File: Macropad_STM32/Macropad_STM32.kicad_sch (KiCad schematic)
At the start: 68 parts, among them J1 USB_C_Receptacle_USB2.0, J10 Encoders + LED, J2 Conn_01x04_Pin, J3 JTAG, J7 Power Connector, J9 Matrix, SW1 SW_Push, U1 STM32F103C8T6, U3 AMS1117-3.3, Y1 16MHz

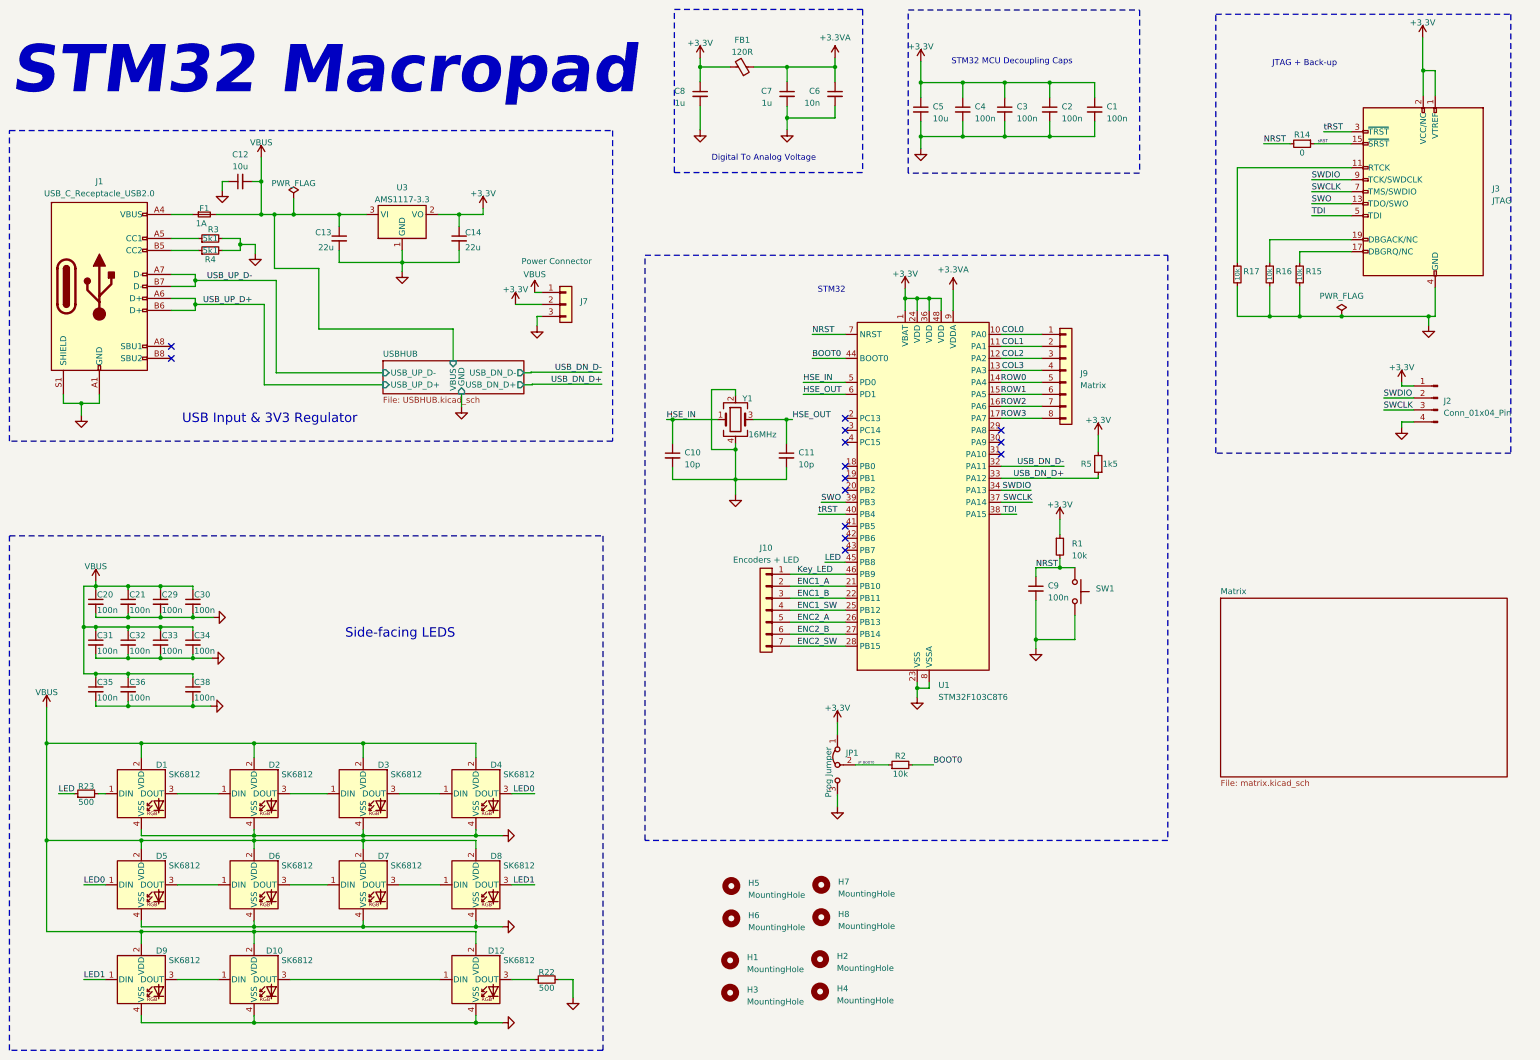
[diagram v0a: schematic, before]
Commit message: Schematic changes Motherboard nearing completion
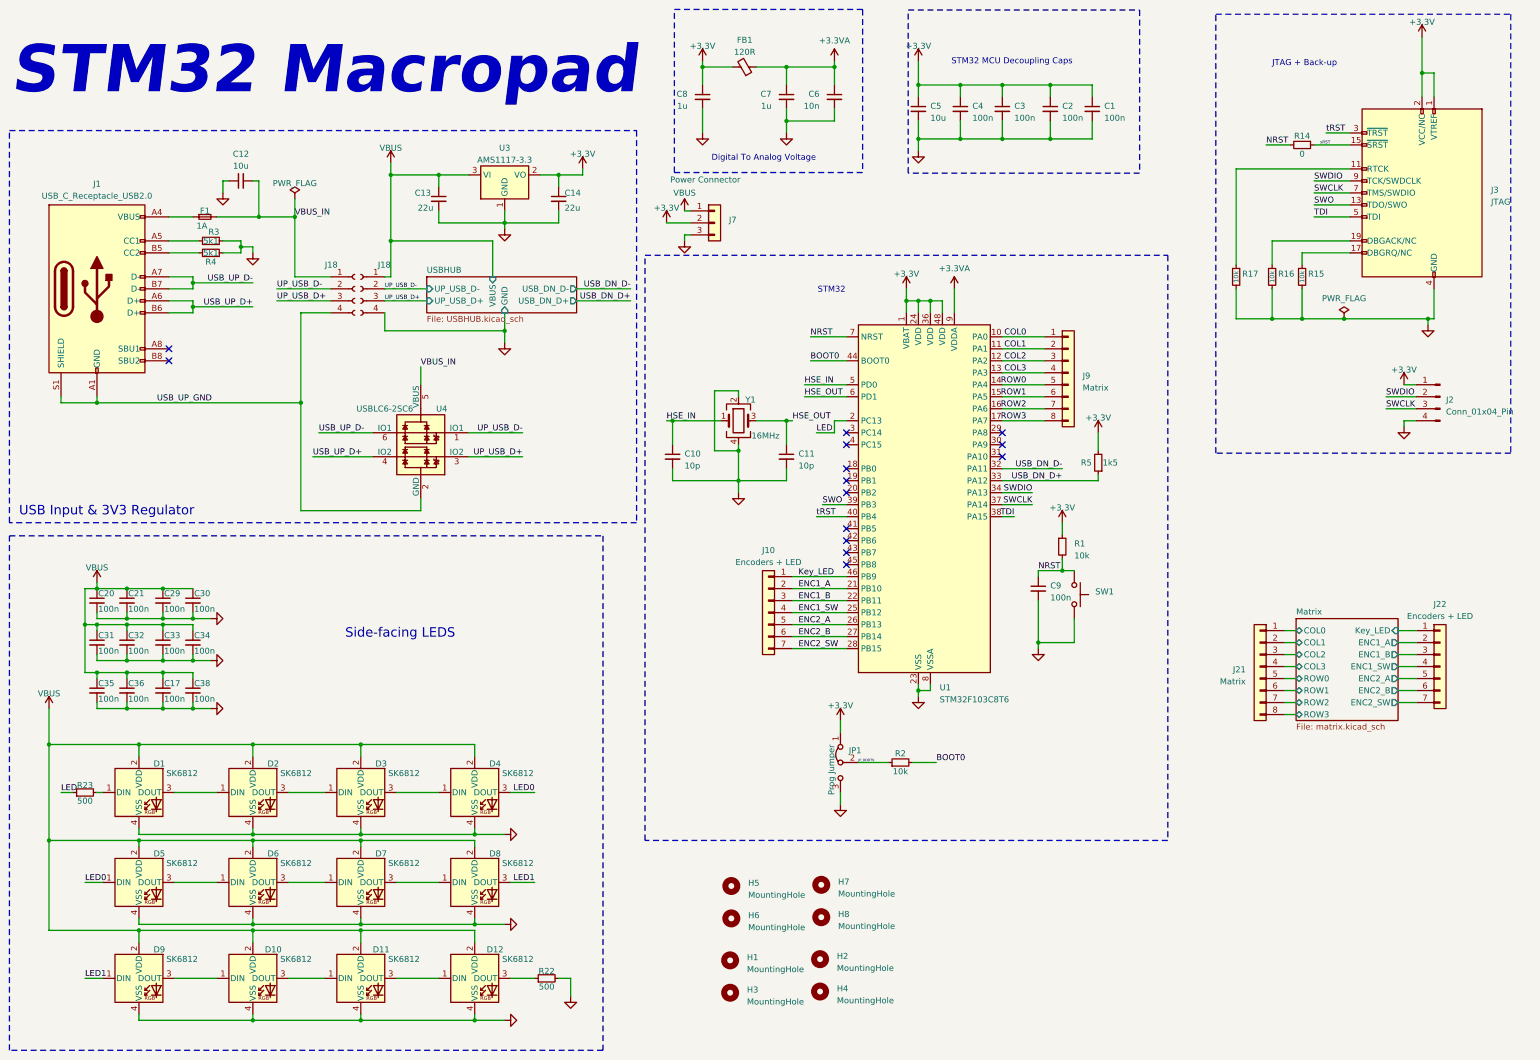
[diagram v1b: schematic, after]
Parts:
- added C17: 100n, Capacitor_SMD:C_0805_2012Metric_Pad1.18x1.45mm_HandSolder, symbol Device:C_Small
- added D11: SK6812, SK6812SIDE:SK6812SIDE, symbol LED:SK6812
- added J18 (x2): Conn_01x04_Socket, Connector_PinHeader_2.54mm:PinHeader_1x04_P2.54mm_Vertical, symbol Connector:Conn_01x04_Socket
- added J21: Matrix, Connector_JST:JST_EH_B8B-EH-A_1x08_P2.50mm_Vertical, symbol Connector_Generic:Conn_01x08
- added J22: Encoders + LED, Connector_JST:JST_EH_B7B-EH-A_1x07_P2.50mm_Vertical, symbol Connector_Generic:Conn_01x07
- added U4: USBLC6-2SC6, Package_TO_SOT_SMD:SOT-23-6, symbol Hub16-rescue:USBLC6-2SC6-josh-ic
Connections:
- net GND: now also C17.2, D11.4 (VSS), J18.4 (Pin_4); no longer J1.A1 (GND), J1.A12 (GND), J1.B1 (GND), J1.B12 (GND), J1.S1 (SHIELD)
- net LED: now also U1.2 (PC13); no longer U1.45 (PB8)
- net USB_UP_D+: now also U4.4 (IO2)
- net USB_UP_D-: now also U4.6 (IO1)
- net VBUS: now also C17.1, D11.2 (VDD), J18.1 (Pin_1); no longer C12.2, F1.2
- net at D10.3 (DOUT): now also D11.1 (DIN); no longer D12.1 (DIN)
- new net: D11.3 (DOUT), D12.1 (DIN)
- new net Matrix/COL0: J21.1 (Pin_1)
- new net Matrix/COL1: J21.2 (Pin_2)
- new net Matrix/COL2: J21.3 (Pin_3)
- new net Matrix/COL3: J21.4 (Pin_4)
- new net Matrix/ENC1_A: J22.2 (Pin_2)
- new net Matrix/ENC1_B: J22.3 (Pin_3)
- new net Matrix/ENC1_SW: J22.4 (Pin_4)
- new net Matrix/ENC2_A: J22.5 (Pin_5)
- new net Matrix/ENC2_B: J22.6 (Pin_6)
- new net Matrix/ENC2_SW: J22.7 (Pin_7)
- new net Matrix/Key_LED: J22.1 (Pin_1)
- new net Matrix/ROW0: J21.5 (Pin_5)
- new net Matrix/ROW1: J21.6 (Pin_6)
- new net Matrix/ROW2: J21.7 (Pin_7)
- new net Matrix/ROW3: J21.8 (Pin_8)
- new net UP_USB_D+: J18.3 (Pin_3), J18.3 (Pin_3), U4.3 (IO2)
- new net UP_USB_D-: J18.2 (Pin_2), J18.2 (Pin_2), U4.1 (IO1)
- new net USB_UP_GND: J1.A1 (GND), J1.A12 (GND), J1.B1 (GND), J1.B12 (GND), J1.S1 (SHIELD), J18.4 (Pin_4), U4.2 (GND)
- new net VBUS_IN: C12.2, F1.2, J18.1 (Pin_1), U4.5 (VBUS)
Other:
- sheet Matrix ports: added COL0, COL1, COL2, COL3, ENC1_A, ENC1_B, ENC1_SW, ENC2_A, ENC2_B, ENC2_SW, Key_LED, ROW0, ROW1, ROW2, ROW3; removed none
- sheet USBHUB ports: added UP_USB_D+, UP_USB_D-; removed USB_UP_D+, USB_UP_D-
- company: (none) -> Irfaan
- moved on the sheet: C1, C13, C14, C29, C3, C33, C4, C5, C6, C7, C8, C9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
